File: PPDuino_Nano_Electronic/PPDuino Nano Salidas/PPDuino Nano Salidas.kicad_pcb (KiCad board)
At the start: 2 copper layers, 51.6 x 92.8 mm, 29 parts, among them J12 OUTPUTS, J13 SEL1, J14 RLY0, J6 SEL0, J7 RLY1, J8 PWM, J9 PWR_OUT, Q1 BC548, Q2 BC548, U5 L293D

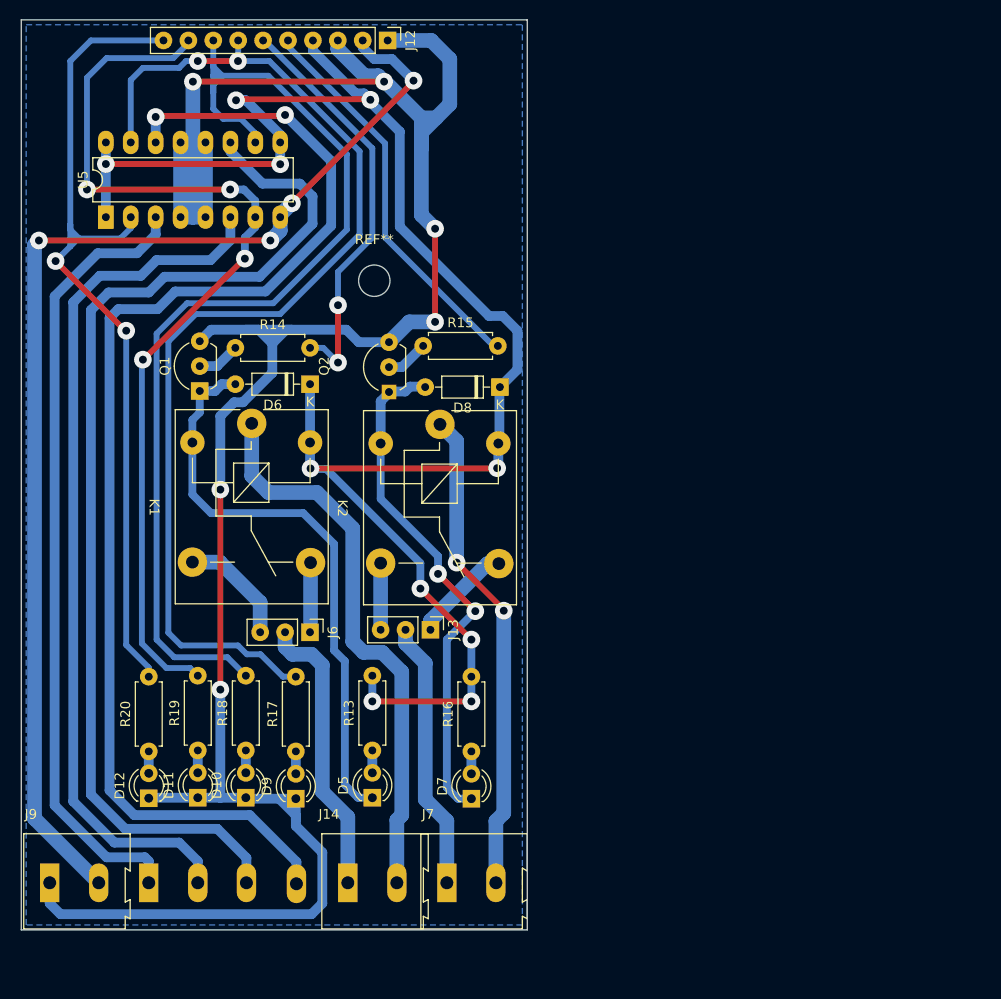
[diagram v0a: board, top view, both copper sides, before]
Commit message: Actualizar documentacion 2
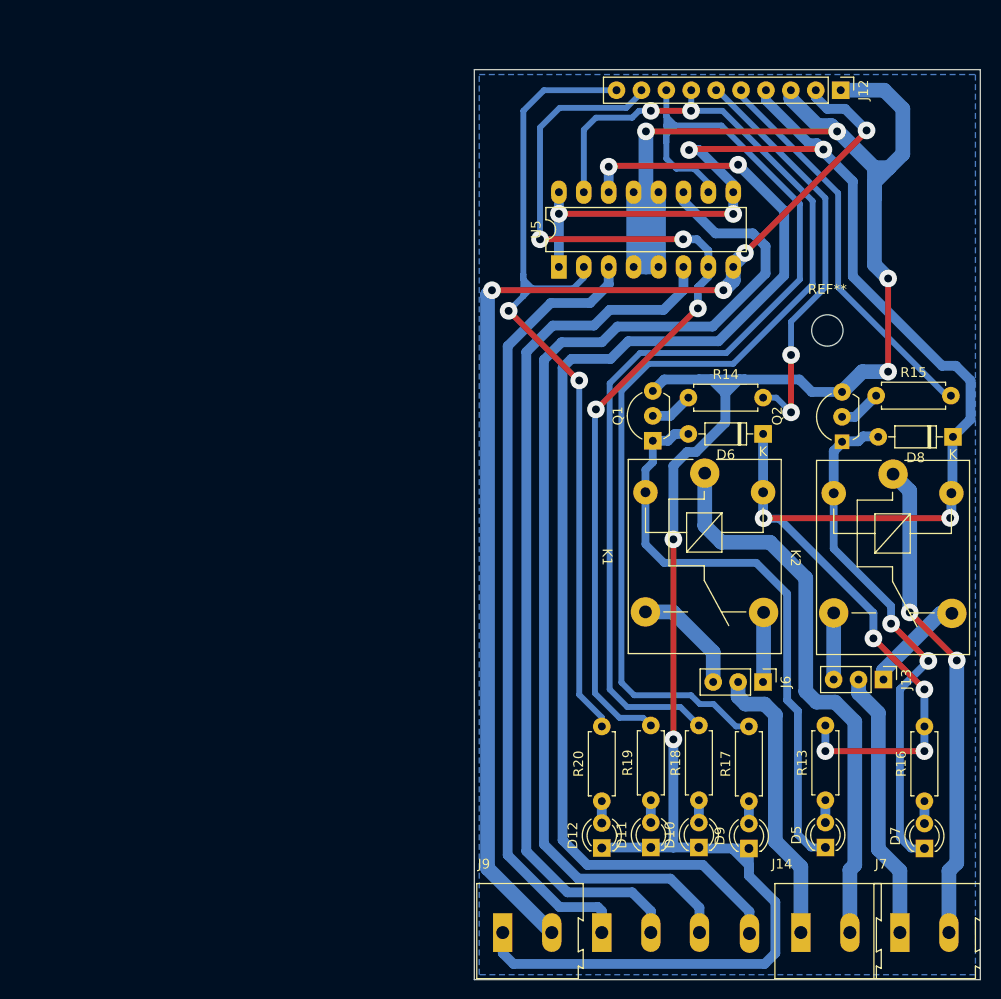
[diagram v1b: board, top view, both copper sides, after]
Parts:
- moved D6 46.5 mm to (147.1, 80.9)
- moved Q1 46.5 mm to (135.8, 81.6)
- moved R15 46.5 mm to (158.6, 77.0)
- moved D10 46.5 mm to (140.5, 123.1)
- moved D5 46.5 mm to (153.4, 123.1)
- moved D7 46.5 mm to (163.5, 123.2)
- moved D8 46.5 mm to (166.4, 81.2)
- moved J12 46.5 mm to (155.0, 45.9)
- moved J14 46.5 mm to (150.9, 131.8)
- moved J7 46.5 mm to (161.0, 131.8)
- moved J8 46.5 mm to (130.6, 131.9)
- moved J9 46.5 mm to (120.5, 131.8)
- moved K1 46.5 mm to (140.8, 93.5)
- moved R13 46.5 mm to (153.4, 118.3)
- moved R14 46.5 mm to (139.4, 77.2)
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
